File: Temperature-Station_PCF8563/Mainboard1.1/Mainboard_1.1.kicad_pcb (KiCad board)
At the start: 2 copper layers, 35 parts, among them J1 CONN_01X03, J2 CONN_01X15, J3 CONN_01X15, J4 SD_Card, J5 CONN_01X03, J6 CONN_01X02, J7 CONN_01X02, J8 CONN_01X02, J9 CONN_01X02, U1 LM1117-3.3, U2 PCF8563, U3 LF33CDT-TR, Y1 Crystal

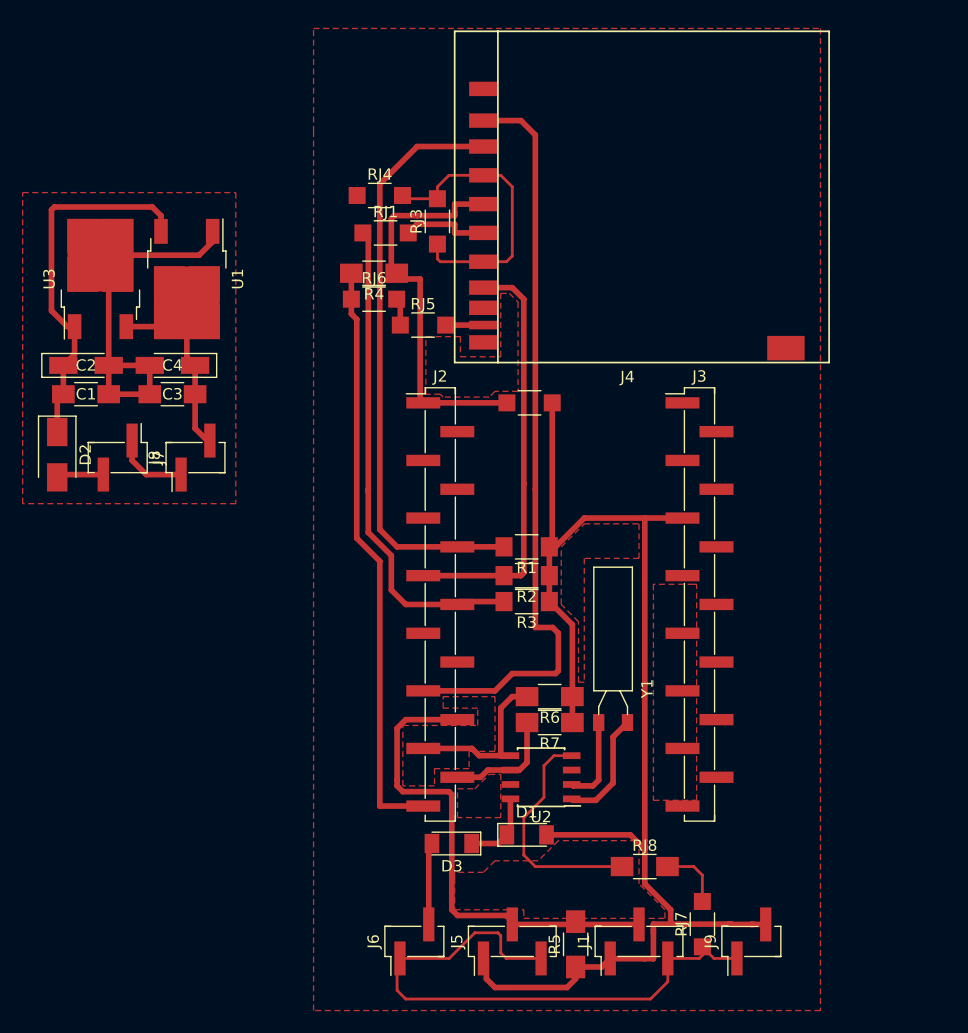
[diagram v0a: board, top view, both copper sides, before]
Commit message: Mainboard changes
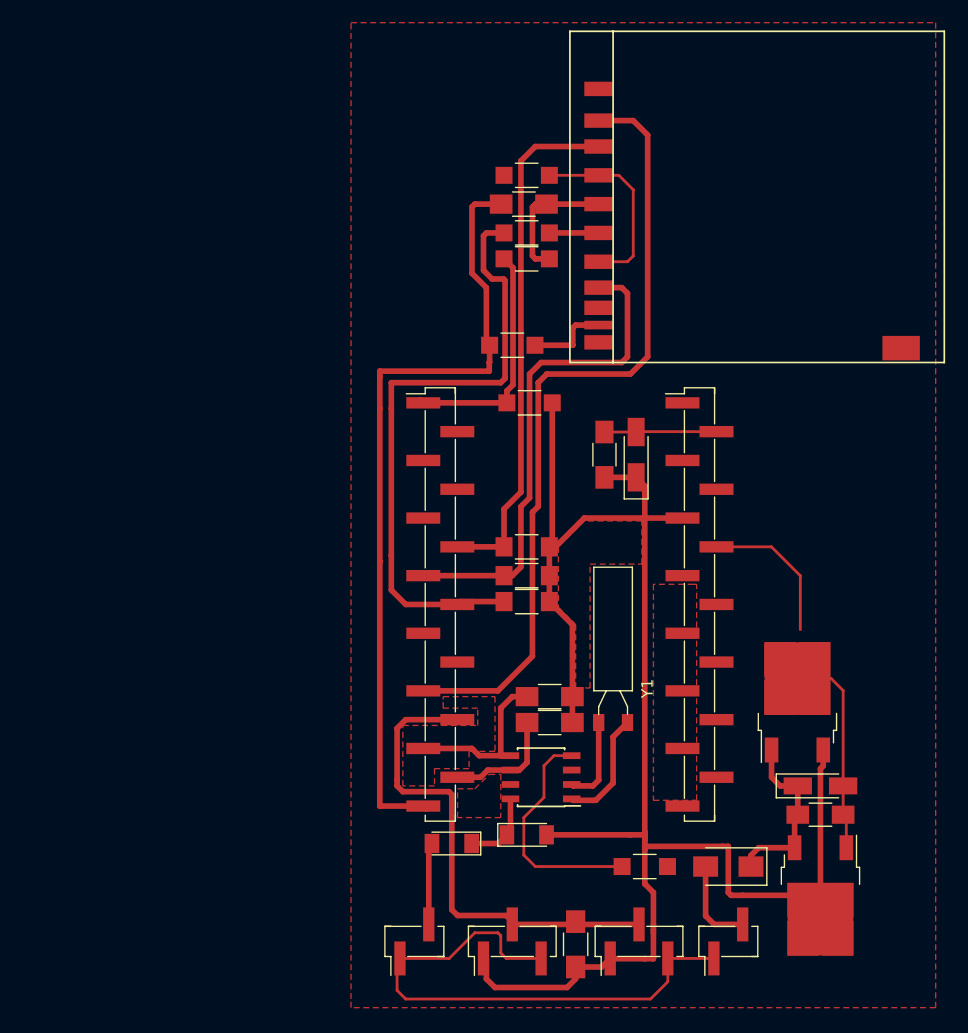
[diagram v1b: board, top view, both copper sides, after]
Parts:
- removed J8, J9: CONN_01X02, Pin_Headers:Pin_Header_Straight_1x02_Pitch2.54mm_SMD_Pin1Left
- removed RJ7, RJ8: 0, Resistors_SMD:R_1206_HandSoldering
- moved U1 78.0 mm to (170.7, 129.8)
- moved C1 74.6 mm to (170.7, 122.7)
- moved C2 74.6 mm to (170.7, 120.1)
- moved U3 71.9 mm to (168.7, 112.8)
- moved D2 69.4 mm to (162.6, 127.3), turned to 180 degrees
- moved J7 68.7 mm to (162.6, 133.9), turned to 90 degrees
- moved RJ6 55.4 mm to (155.2, 127.3)
- moved C4 41.6 mm to (154.4, 90.9), turned to 90 degrees
- moved C3 38.5 mm to (151.6, 90.9), turned to 90 degrees
- moved R4 14.5 mm to (144.5, 68.8)
- moved RJ4 13.1 mm to (144.8, 66.3)
- moved RJ1 12.4 mm to (144.8, 71.4)
- moved J4 10.2 mm to (172.7, 62.5)
- moved RJ3 8.54 mm to (144.8, 73.7), turned to 180 degrees
- moved RJ5 8.07 mm to (143.5, 81.3)
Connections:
- C1 pad 2: Net-(C1-Pad2) -> GND
- C2 pad 2: Net-(C1-Pad2) -> GND
- C3 pad 1: Net-(C3-Pad1) -> 3V3
- C3 pad 2: Net-(C1-Pad2) -> GND
- C4 pad 1: Net-(C3-Pad1) -> 3V3
- C4 pad 2: Net-(C1-Pad2) -> GND
- J7 pad 1: Net-(C1-Pad2) -> GND
- RJ3 pad 1: GND -> 3V3
- RJ3 pad 2: GND -> 3V3
- RJ5 pad 1: Net-(RJ5-Pad1) -> SD_D
- RJ6 pad 1: SD_D -> GND
- RJ6 pad 2: Net-(RJ5-Pad1) -> GND
- U1 pad 1: Net-(C1-Pad2) -> GND
- U1 pad 2: Net-(C3-Pad1) -> 3V3
- U3 pad 2: Net-(C1-Pad2) -> GND
- U3 pad 3: Net-(C3-Pad1) -> 3V3
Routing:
- net Net-(C1-Pad2): track 41.0 -> 0.00 mm
- net 3V3: track 157.8 -> 185.8 mm
- net GND: track 105.6 -> 129.1 mm
- net Net-(C3-Pad1): track 19.3 -> 0.00 mm
- net SD_D: track 52.5 -> 70.1 mm
- net Net-(C1-Pad1): track 33.1 -> 15.7 mm
- net Net-(J2-Pad8): track 43.8 -> 54.9 mm
- net MISO: track 37.1 -> 43.9 mm
- net MOSI: track 52.6 -> 46.2 mm
- net Net-(J4-Pad10): track 3.33 -> 7.25 mm
- net Net-(D2-Pad2): track 4.17 -> 7.93 mm
- net SCK: track 7.71 -> 4.10 mm
- net CS: track 66.7 -> 70.2 mm
- net Net-(RJ5-Pad1): track 3.32 -> 0.00 mm
- removed copper zone on F.Cu, net Net-(C1-Pad2)
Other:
- board text added: "C2"
- board text added: "C3"
